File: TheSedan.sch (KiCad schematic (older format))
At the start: 152 parts, among them SW1 SW_Push, U2 ATmega32U4-AU, Y1 16MHz

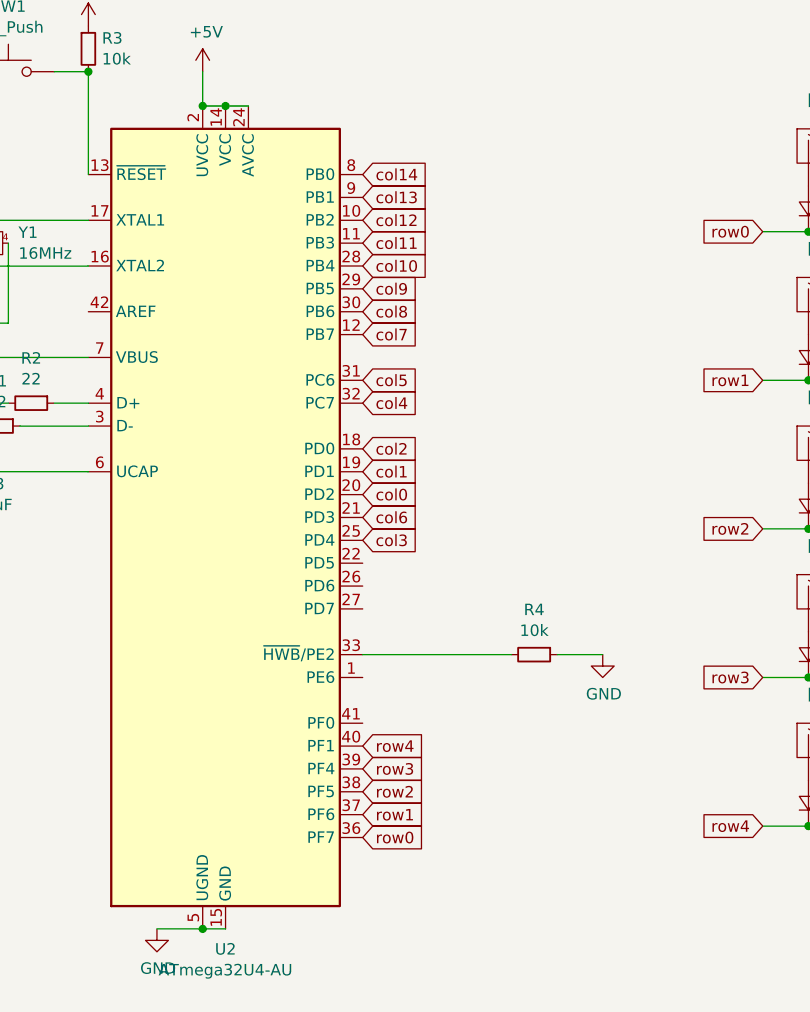
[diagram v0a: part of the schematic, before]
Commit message: 5/4/20 v3
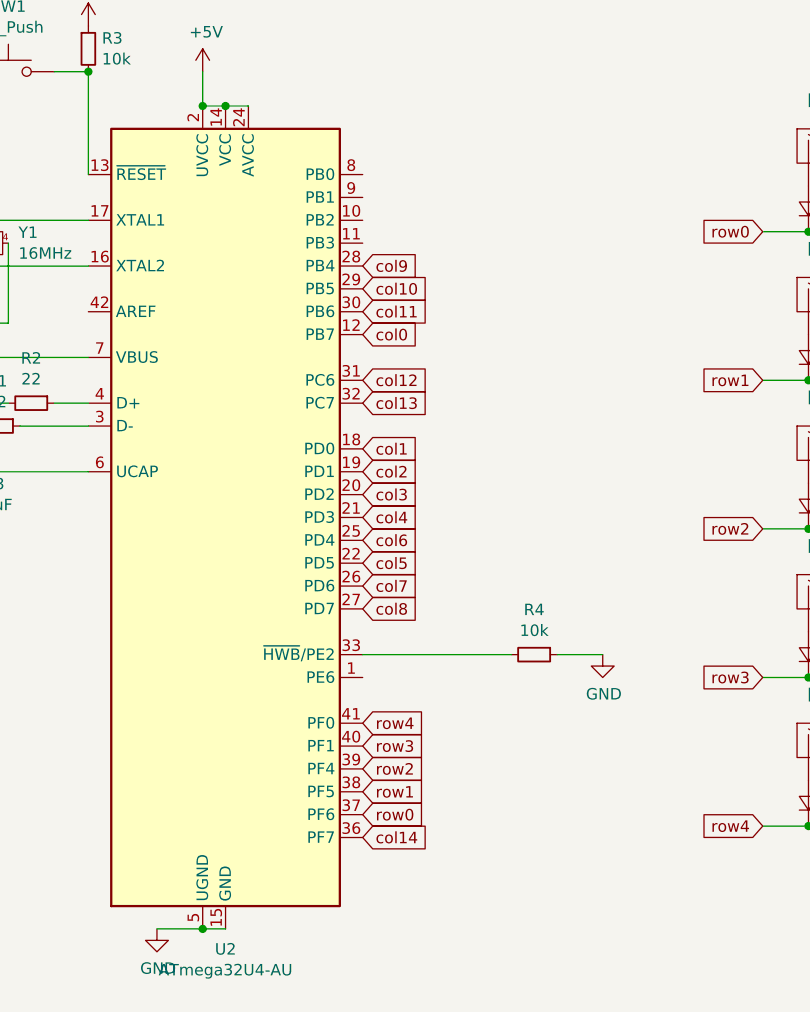
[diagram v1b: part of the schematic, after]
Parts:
- F1: footprint Fuse:Fuse_1206_3216Metric -> Fuse:Fuse_1210_3225Metric
- USB1: footprint random-keyboard-parts:Molex-0548190589 -> Connector_USB:USB_Micro-B_Molex_47346-0001
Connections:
- net col0: now also U2.12 (PB7); no longer U2.20 (PD2)
- net col1: now also U2.18 (PD0); no longer U2.19 (PD1)
- net col10: now also U2.29 (PB5); no longer U2.28 (PB4)
- net col11: now also U2.30 (PB6); no longer U2.11 (PB3)
- net col12: now also U2.31 (PC6); no longer U2.10 (PB2)
- net col13: now also U2.32 (PC7); no longer U2.9 (PB1)
- net col14: now also U2.36 (PF7); no longer U2.8 (PB0)
- net col2: now also U2.19 (PD1); no longer U2.18 (PD0)
- net col3: now also U2.20 (PD2); no longer U2.25 (PD4)
- net col4: now also U2.21 (PD3); no longer U2.32 (PC7)
- net col5: now also U2.22 (PD5); no longer U2.31 (PC6)
- net col6: now also U2.25 (PD4); no longer U2.21 (PD3)
- net col7: now also U2.26 (PD6); no longer U2.12 (PB7)
- net col8: now also U2.27 (PD7); no longer U2.30 (PB6)
- net col9: now also U2.28 (PB4); no longer U2.29 (PB5)
- net row0: now also U2.37 (PF6); no longer U2.36 (PF7)
- net row1: now also U2.38 (PF5); no longer U2.37 (PF6)
- net row2: now also U2.39 (PF4); no longer U2.38 (PF5)
- net row3: now also U2.40 (PF1); no longer U2.39 (PF4)
- net row4: now also U2.41 (PF0); no longer U2.40 (PF1)
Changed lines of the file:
@@
 Text GLabel 11000 900  1    50   Input ~ 0
 col14
+Text GLabel 2550 3300 2    50   Input ~ 0
+col8
+Text GLabel 2550 1800 2    50   Input ~ 0
+col9
+Text GLabel 2550 1900 2    50   Input ~ 0
+col10
 Text GLabel 2550 2000 2    50   Input ~ 0
-col8
-Text GLabel 2550 1900 2    50   Input ~ 0
-col9
-Text GLabel 2550 1800 2    50   Input ~ 0
-col10
-Text GLabel 2550 1700 2    50   Input ~ 0
 col11
-Text GLabel 2550 1600 2    50   Input ~ 0
+Text GLabel 2550 2300 2    50   Input ~ 0
 col12
-Text GLabel 2550 1500 2    50   Input ~ 0
+Text GLabel 2550 2400 2    50   Input ~ 0
 col13
-Text GLabel 2550 1400 2    50   Input ~ 0
+Text GLabel 2550 4300 2    50   Input ~ 0
 col14
 Text GLabel 4300 2300 0    50   Input ~ 0
@@
 Text GLabel 4300 4250 0    50   Input ~ 0
 row4
+Text GLabel 2550 4100 2    50   Input ~ 0
+row1
 Text GLabel 2550 4200 2    50   Input ~ 0
-row1
-Text GLabel 2550 4300 2    50   Input ~ 0
 row0
-Text GLabel 2550 4100 2    50   Input ~ 0
+Text GLabel 2550 4000 2    50   Input ~ 0
 row2
-Text GLabel 2550 4000 2    50   Input ~ 0
+Text GLabel 2550 3900 2    50   Input ~ 0
 row3
-Text GLabel 2550 3900 2    50   Input ~ 0
+Text GLabel 2550 3800 2    50   Input ~ 0
 row4
 Wire Wire Line
@@
 Wire Wire Line
 	11000 3200 11000 3850
-Text GLabel 2550 2100 2    50   Input ~ 0
+Text GLabel 2550 3200 2    50   Input ~ 0
 col7
+Text GLabel 2550 3000 2    50   Input ~ 0
+col6
+Text GLabel 2550 3100 2    50   Input ~ 0
+col5
 Text GLabel 2550 2900 2    50   Input ~ 0
-col6
-Text GLabel 2550 2300 2    50   Input ~ 0
-col5
-Text GLabel 2550 2400 2    50   Input ~ 0
 col4
-Text GLabel 2550 3000 2    50   Input ~ 0
+Text GLabel 2550 2800 2    50   Input ~ 0
 col3
+Text GLabel 2550 2700 2    50   Input ~ 0
+col2
 Text GLabel 2550 2600 2    50   Input ~ 0
-col2
-Text GLabel 2550 2700 2    50   Input ~ 0
 col1
-Text GLabel 2550 2800 2    50   Input ~ 0
-col0
 $Comp
 L MCU_Microchip_ATmega:ATmega32U4-AU U2
@@
 Text GLabel 650  2500 0    50   Input ~ 0
 D-
-$Comp
-L random-keyboard-parts:Molex-0548190589 USB1
-U 1 1 5EC9EE94
-P 3300 5950
-F 0 "USB1" V 3837 5917 60  0000 C CNN
-F 1 "Molex-0548190589" V 3731 5917 60  0000 C CNN
-F 2 "random-keyboard-parts:Molex-0548190589" H 3300 5950 60  0001 C CNN
-F 3 "" H 3300 5950 60  0001 C CNN
-	1    3300 5950
-	0    -1   -1   0
-$EndComp
 Text GLabel 3650 5950 2    50   Input ~ 0
 D+
@@
 	3900 5750 4050 5750
 $Comp
-L Device:Polyfuse_Small F1
-U 1 1 5ECDBA70
-P 4150 5750
-F 0 "F1" V 3945 5750 50  0000 C CNN
-F 1 "500mA" V 4036 5750 50  0000 C CNN
-F 2 "Fuse:Fuse_1206_3216Metric" H 4200 5550 50  0001 L CNN
-F 3 "~" H 4150 5750 50  0001 C CNN
-	1    4150 5750
-	0    1    1    0
-$EndComp
-$Comp
 L power:+5V #PWR0113
 U 1 1 5ED01E32
@@
 Wire Wire Line
 	4250 5750 4400 5750
+$Comp
+L random-keyboard-parts:Molex-0548190589 USB1
+U 1 1 5EC9EE94
+P 3300 5950
+F 0 "USB1" V 3837 5917 60  0000 C CNN
+F 1 "Molex-0548190589" V 3731 5917 60  0000 C CNN
+F 2 "Connector_USB:USB_Micro-B_Molex_47346-0001" H 3300 5950 60  0001 C CNN
+F 3 "" H 3300 5950 60  0001 C CNN
+	1    3300 5950
+	0    -1   -1   0
+$EndComp
+Text GLabel 2550 2100 2    50   Input ~ 0
+col0
+$Comp
+L Device:Polyfuse_Small F1
+U 1 1 5ECDBA70
+P 4150 5750
+F 0 "F1" V 3945 5750 50  0000 C CNN
+F 1 "500mA" V 4036 5750 50  0000 C CNN
+F 2 "Fuse:Fuse_1210_3225Metric" H 4200 5550 50  0001 L CNN
+F 3 "~" H 4150 5750 50  0001 C CNN
+	1    4150 5750
+	0    1    1    0
+$EndComp
 $EndSCHEMATC

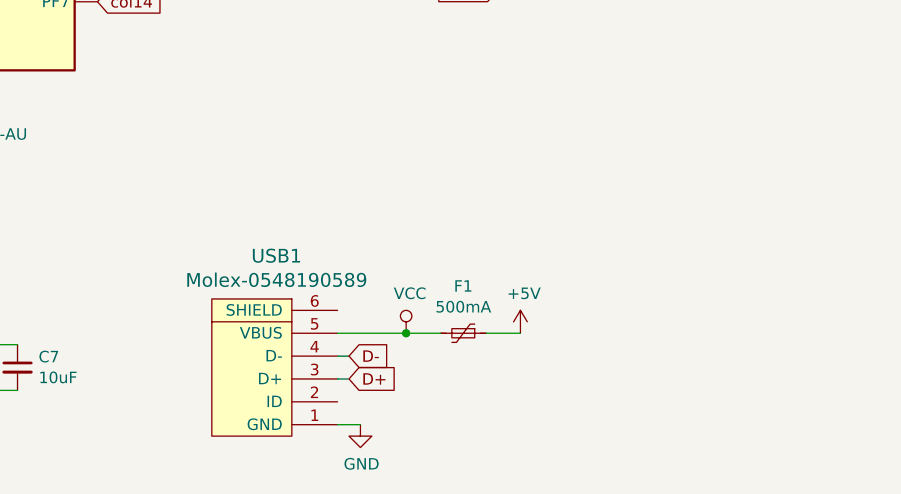
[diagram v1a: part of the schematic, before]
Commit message: 5/4/20 v3
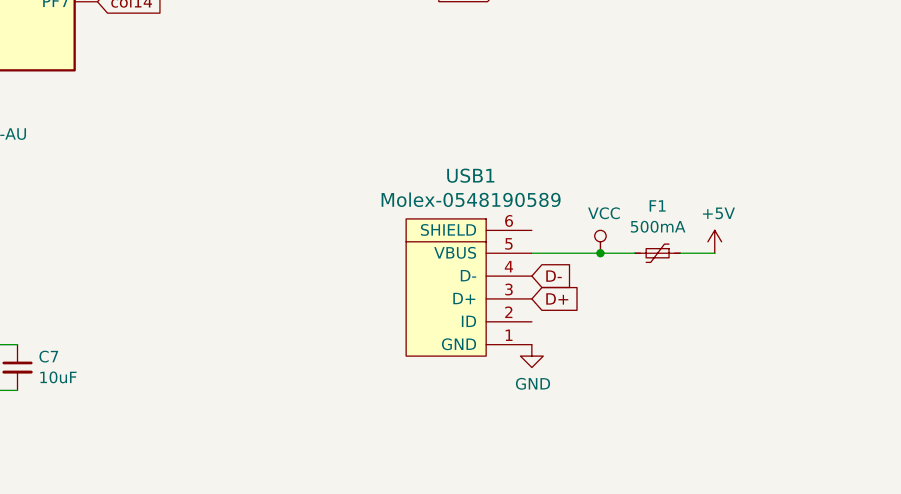
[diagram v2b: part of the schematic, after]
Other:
- moved on the sheet: F1, USB1
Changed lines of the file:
@@
 Text GLabel 650  2500 0    50   Input ~ 0
 D-
-Text GLabel 3650 5950 2    50   Input ~ 0
+Text GLabel 4450 5600 2    50   Input ~ 0
 D+
-Wire Wire Line
-	3600 5950 3650 5950
-Text GLabel 3650 5850 2    50   Input ~ 0
+Text GLabel 4450 5500 2    50   Input ~ 0
 D-
-Wire Wire Line
-	3600 5850 3650 5850
 $Comp
 L power:GND #PWR0111
 U 1 1 5ECB670F
-P 3700 6150
-F 0 "#PWR0111" H 3700 5900 50  0001 C CNN
-F 1 "GND" H 3705 5977 50  0000 C CNN
-F 2 "" H 3700 6150 50  0001 C CNN
-F 3 "" H 3700 6150 50  0001 C CNN
-	1    3700 6150
+P 4450 5800
+F 0 "#PWR0111" H 4450 5550 50  0001 C CNN
+F 1 "GND" H 4455 5627 50  0000 C CNN
+F 2 "" H 4450 5800 50  0001 C CNN
+F 3 "" H 4450 5800 50  0001 C CNN
+	1    4450 5800
 	1    0    0    -1
 $EndComp
 Wire Wire Line
-	3600 6150 3700 6150
-Wire Wire Line
-	3600 5750 3900 5750
+	4450 5400 4750 5400
 $Comp
 L power:VCC #PWR0112
 U 1 1 5ECCB698
-P 3900 5750
-F 0 "#PWR0112" H 3900 5600 50  0001 C CNN
-F 1 "VCC" H 3917 5923 50  0000 C CNN
-F 2 "" H 3900 5750 50  0001 C CNN
-F 3 "" H 3900 5750 50  0001 C CNN
-	1    3900 5750
+P 4750 5400
+F 0 "#PWR0112" H 4750 5250 50  0001 C CNN
+F 1 "VCC" H 4767 5573 50  0000 C CNN
+F 2 "" H 4750 5400 50  0001 C CNN
+F 3 "" H 4750 5400 50  0001 C CNN
+	1    4750 5400
 	1    0    0    -1
 $EndComp
-Connection ~ 3900 5750
+Connection ~ 4750 5400
 Wire Wire Line
-	3900 5750 4050 5750
+	4750 5400 4900 5400
 $Comp
 L power:+5V #PWR0113
 U 1 1 5ED01E32
-P 4400 5750
-F 0 "#PWR0113" H 4400 5600 50  0001 C CNN
-F 1 "+5V" H 4415 5923 50  0000 C CNN
-F 2 "" H 4400 5750 50  0001 C CNN
-F 3 "" H 4400 5750 50  0001 C CNN
-	1    4400 5750
+P 5250 5400
+F 0 "#PWR0113" H 5250 5250 50  0001 C CNN
+F 1 "+5V" H 5265 5573 50  0000 C CNN
+F 2 "" H 5250 5400 50  0001 C CNN
+F 3 "" H 5250 5400 50  0001 C CNN
+	1    5250 5400
 	1    0    0    -1
 $EndComp
 Wire Wire Line
-	4250 5750 4400 5750
+	5100 5400 5250 5400
 $Comp
 L random-keyboard-parts:Molex-0548190589 USB1
 U 1 1 5EC9EE94
-P 3300 5950
-F 0 "USB1" V 3837 5917 60  0000 C CNN
-F 1 "Molex-0548190589" V 3731 5917 60  0000 C CNN
-F 2 "Connector_USB:USB_Micro-B_Molex_47346-0001" H 3300 5950 60  0001 C CNN
-F 3 "" H 3300 5950 60  0001 C CNN
-	1    3300 5950
+P 4150 5600
+F 0 "USB1" V 4687 5567 60  0000 C CNN
+F 1 "Molex-0548190589" V 4581 5567 60  0000 C CNN
+F 2 "Connector_USB:USB_Micro-B_Molex_47346-0001" H 4150 5600 60  0001 C CNN
+F 3 "" H 4150 5600 60  0001 C CNN
+	1    4150 5600
 	0    -1   -1   0
 $EndComp
@@
 L Device:Polyfuse_Small F1
 U 1 1 5ECDBA70
-P 4150 5750
-F 0 "F1" V 3945 5750 50  0000 C CNN
-F 1 "500mA" V 4036 5750 50  0000 C CNN
-F 2 "Fuse:Fuse_1210_3225Metric" H 4200 5550 50  0001 L CNN
-F 3 "~" H 4150 5750 50  0001 C CNN
-	1    4150 5750
+P 5000 5400
+F 0 "F1" V 4795 5400 50  0000 C CNN
+F 1 "500mA" V 4886 5400 50  0000 C CNN
+F 2 "Fuse:Fuse_1210_3225Metric" H 5050 5200 50  0001 L CNN
+F 3 "~" H 5000 5400 50  0001 C CNN
+	1    5000 5400
 	0    1    1    0
 $EndComp

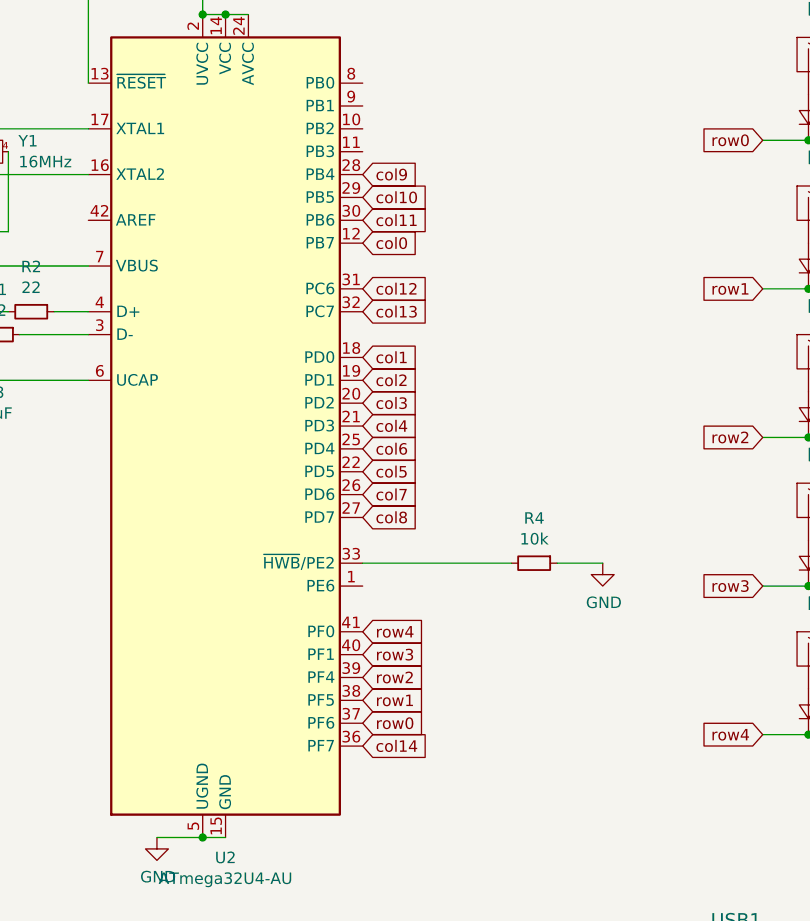
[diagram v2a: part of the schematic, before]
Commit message: 5/5/20 v1
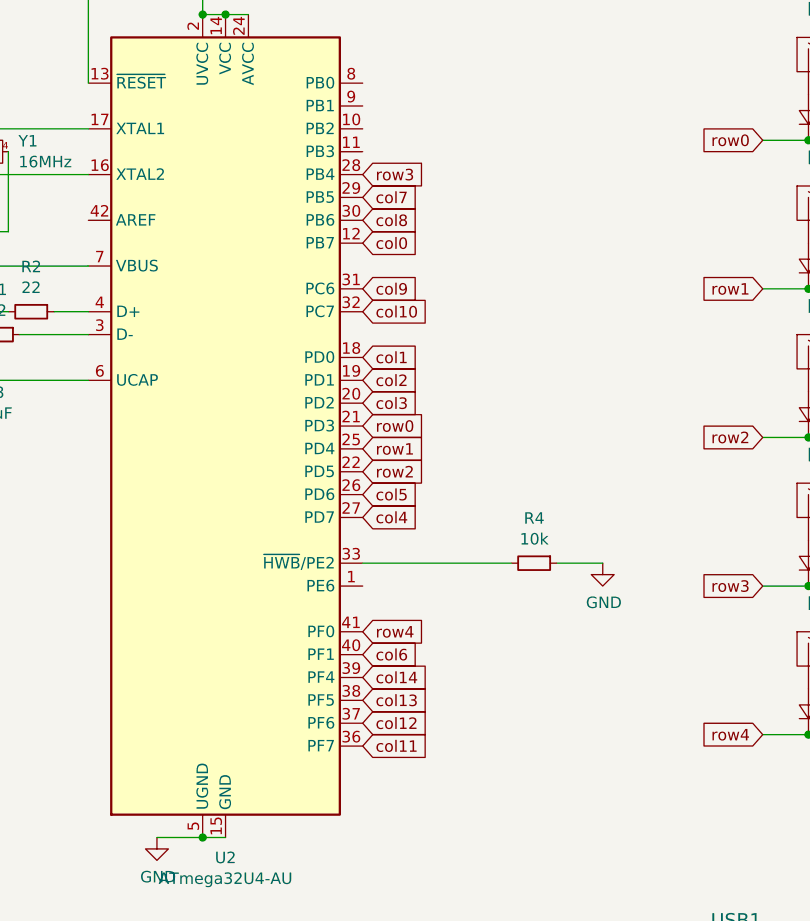
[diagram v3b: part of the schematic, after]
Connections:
- net col10: now also U2.32 (PC7); no longer U2.29 (PB5)
- net col11: now also U2.36 (PF7); no longer U2.30 (PB6)
- net col12: now also U2.37 (PF6); no longer U2.31 (PC6)
- net col13: now also U2.38 (PF5); no longer U2.32 (PC7)
- net col14: now also U2.39 (PF4); no longer U2.36 (PF7)
- net col4: now also U2.27 (PD7); no longer U2.21 (PD3)
- net col5: now also U2.26 (PD6); no longer U2.22 (PD5)
- net col6: now also U2.40 (PF1); no longer U2.25 (PD4)
- net col7: now also U2.29 (PB5); no longer U2.26 (PD6)
- net col8: now also U2.30 (PB6); no longer U2.27 (PD7)
- net col9: now also U2.31 (PC6); no longer U2.28 (PB4)
- net row0: now also U2.21 (PD3); no longer U2.37 (PF6)
- net row1: now also U2.25 (PD4); no longer U2.38 (PF5)
- net row2: now also U2.22 (PD5); no longer U2.39 (PF4)
- net row3: now also U2.28 (PB4); no longer U2.40 (PF1)
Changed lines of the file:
@@
 Text GLabel 11000 900  1    50   Input ~ 0
 col14
-Text GLabel 2550 3300 2    50   Input ~ 0
+Text GLabel 2550 2000 2    50   Input ~ 0
 col8
-Text GLabel 2550 1800 2    50   Input ~ 0
+Text GLabel 2550 2300 2    50   Input ~ 0
 col9
-Text GLabel 2550 1900 2    50   Input ~ 0
+Text GLabel 2550 2400 2    50   Input ~ 0
 col10
-Text GLabel 2550 2000 2    50   Input ~ 0
+Text GLabel 2550 4300 2    50   Input ~ 0
 col11
-Text GLabel 2550 2300 2    50   Input ~ 0
+Text GLabel 2550 4200 2    50   Input ~ 0
 col12
-Text GLabel 2550 2400 2    50   Input ~ 0
+Text GLabel 2550 4100 2    50   Input ~ 0
 col13
-Text GLabel 2550 4300 2    50   Input ~ 0
+Text GLabel 2550 4000 2    50   Input ~ 0
 col14
 Text GLabel 4300 2300 0    50   Input ~ 0
@@
 Text GLabel 4300 4250 0    50   Input ~ 0
 row4
-Text GLabel 2550 4100 2    50   Input ~ 0
+Text GLabel 2550 3000 2    50   Input ~ 0
 row1
-Text GLabel 2550 4200 2    50   Input ~ 0
+Text GLabel 2550 2900 2    50   Input ~ 0
 row0
-Text GLabel 2550 4000 2    50   Input ~ 0
+Text GLabel 2550 3100 2    50   Input ~ 0
 row2
-Text GLabel 2550 3900 2    50   Input ~ 0
+Text GLabel 2550 1800 2    50   Input ~ 0
 row3
 Text GLabel 2550 3800 2    50   Input ~ 0
@@
 Wire Wire Line
 	11000 3200 11000 3850
+Text GLabel 2550 1900 2    50   Input ~ 0
+col7
+Text GLabel 2550 3900 2    50   Input ~ 0
+col6
 Text GLabel 2550 3200 2    50   Input ~ 0
-col7
-Text GLabel 2550 3000 2    50   Input ~ 0
-col6
-Text GLabel 2550 3100 2    50   Input ~ 0
 col5
-Text GLabel 2550 2900 2    50   Input ~ 0
+Text GLabel 2550 3300 2    50   Input ~ 0
 col4
 Text GLabel 2550 2800 2    50   Input ~ 0
